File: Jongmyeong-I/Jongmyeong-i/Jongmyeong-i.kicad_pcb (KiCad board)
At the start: 2 copper layers, 88 x 56.4 mm, 46 parts, among them J1 Screw3, J11 Screw3, J12 xt30, J13 Screw_Terminal_01x02, J14 Screw_Terminal_01x02, J2 Screw3, J3 Screw3, J4 Screw3, J5 Screw3, J6 Conn_01x03_Pin, J7 Conn_01x08_Pin, J8 Conn_01x03_Pin, J9 Screw3, SW2 SW_DPDT_x2

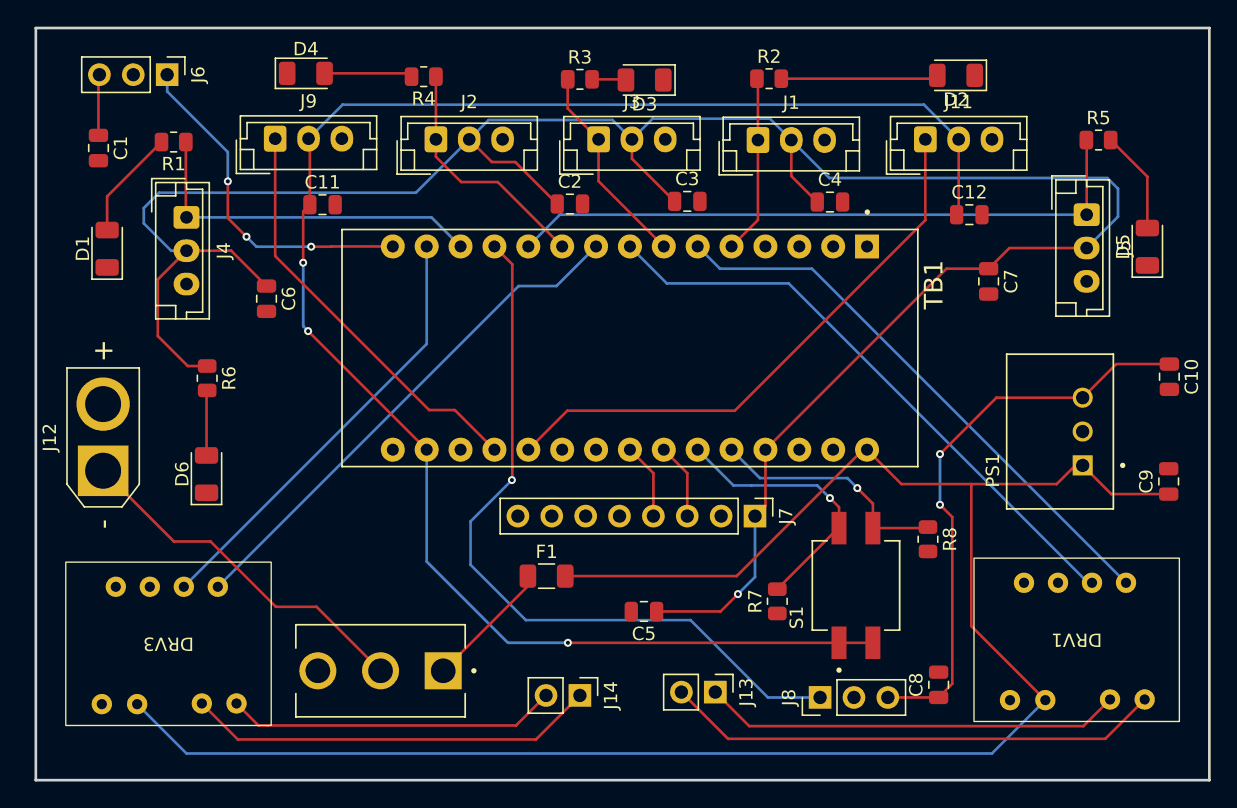
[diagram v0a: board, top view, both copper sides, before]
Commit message: mom
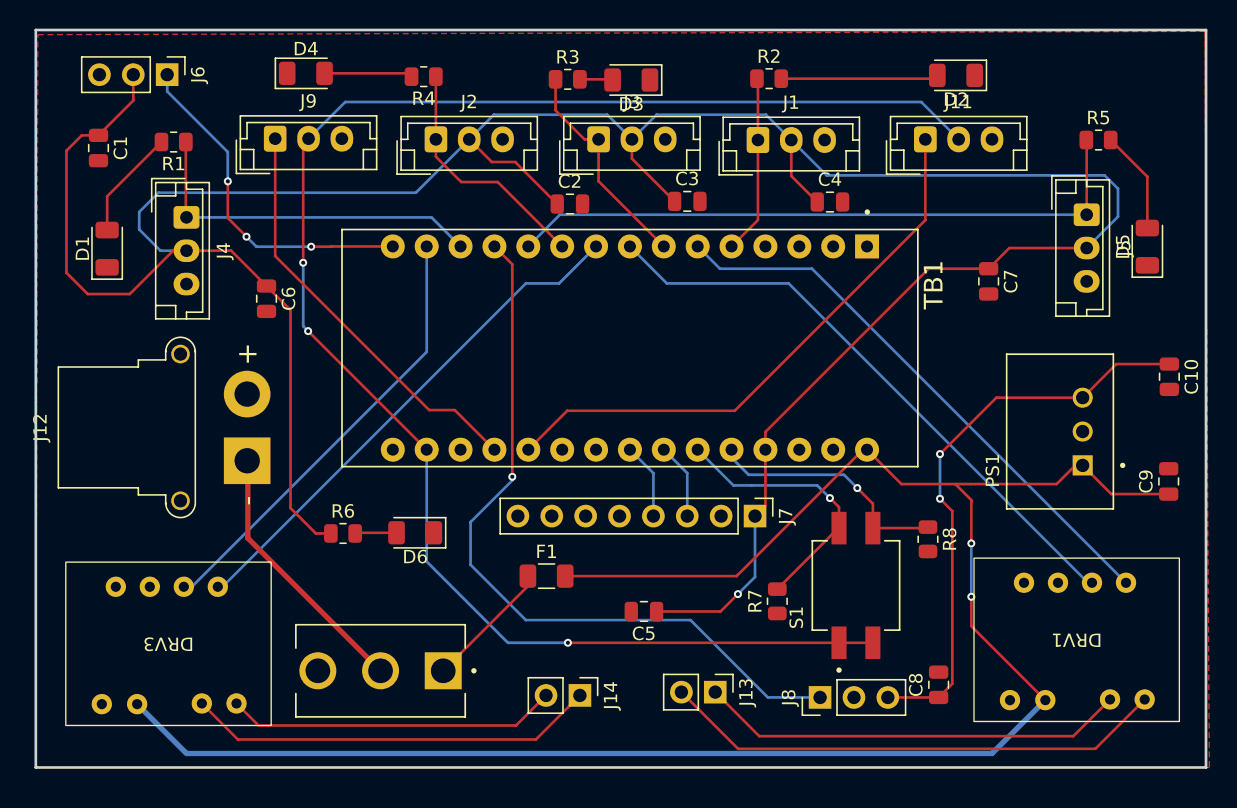
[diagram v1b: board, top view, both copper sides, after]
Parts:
- removed C11, C12: 0.1uF, Capacitor_SMD:C_0805_2012Metric
- J12: footprint Connector_AMASS:AMASS_XT30U-F_1x02_P5.0mm_Vertical -> Connector_AMASS:AMASS_XT30PW-F_1x02_P2.50mm_Horizontal
- moved D6 16.3 mm to (135.3, 100.8), turned to 180 degrees
- moved R6 15.5 mm to (129.9, 100.8), turned to 0 degrees
- moved J12 10.8 mm to (122.7, 95.4)
- moved D3 1.00 mm to (151.5, 66.8)
- moved R3 0.91 mm to (146.7, 66.8)
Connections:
- J6 pad 2: GND -> +5V
- J6 pad 3: +5V -> GND
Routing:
- net +5V: track 182.1 -> 217.7 mm
- net Net-(J12-Pin_1): track 27.0 -> 19.9 mm
- net +3.3V: track 128.4 -> 122.7 mm
- net Net-(D6-A): track 4.83 -> 3.12 mm
- net S2: track 15.5 -> 16.5 mm
- net Net-(DRV1-Out1): track 37.4 -> 38.0 mm
- net Net-(DRV1-Out2): track 31.5 -> 32.1 mm
- net +12V: track 141.5 -> 142.0 mm, vias 0 -> 2
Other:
- board size 88 x 56.4 mm -> 87.8 x 55.3 mm
- board text removed: "${REFERENCE}"
